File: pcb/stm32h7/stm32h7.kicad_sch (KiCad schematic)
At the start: 39 parts, among them J6 Test Pads, SW1 SW_Push, SW2 SW_Push, SW3 SW_Push, U1 STM32H743VGTx, U11 TPS61169DCKR, U9 MT25QUxxxxxx1xW7, Y1 25MHz

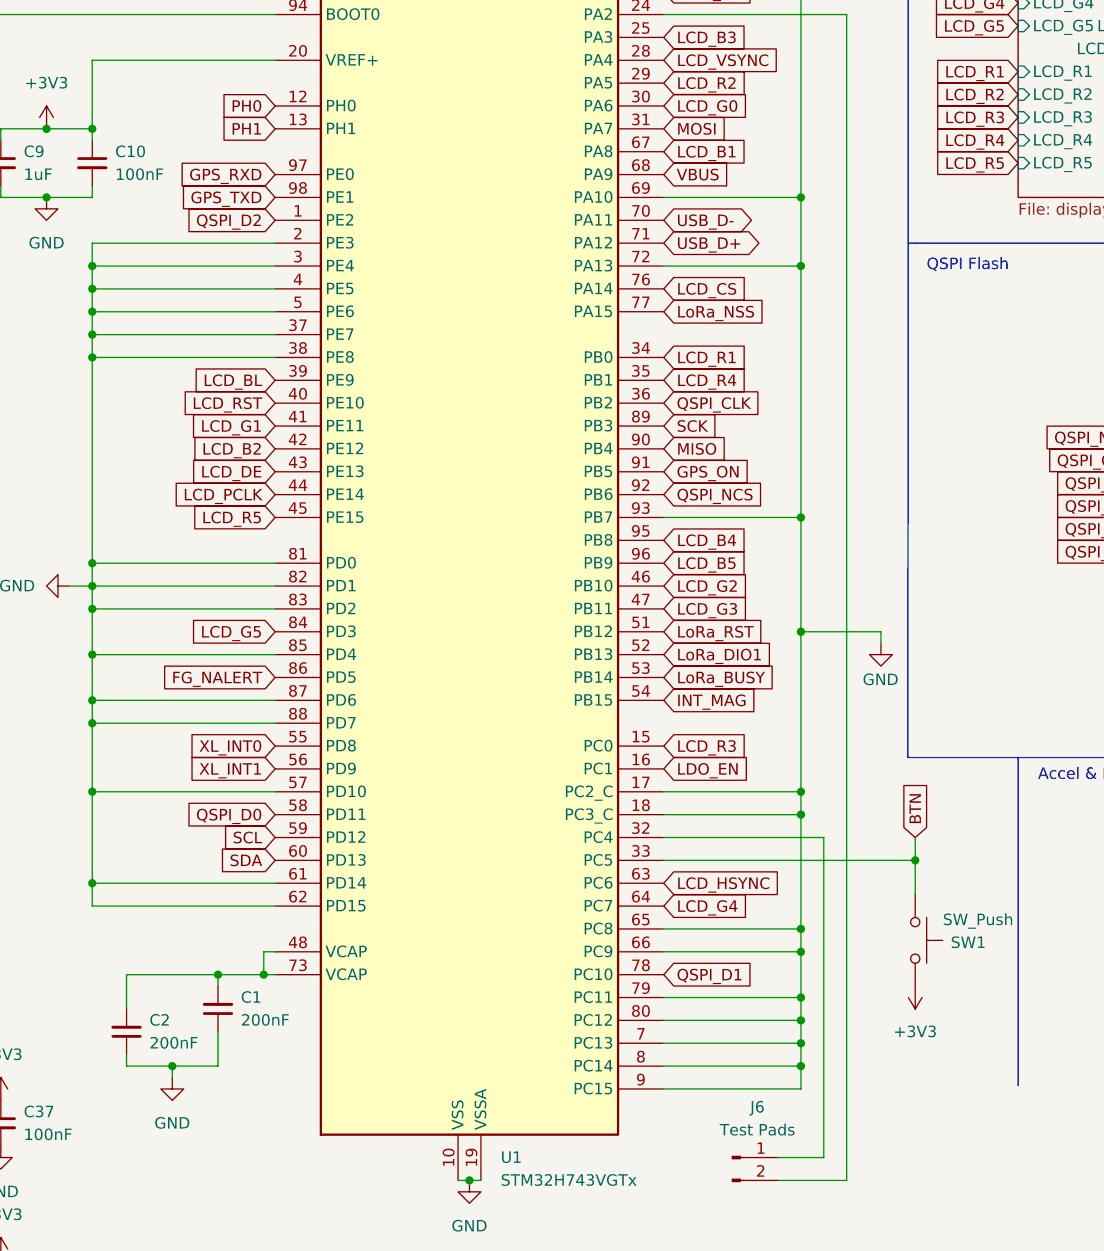
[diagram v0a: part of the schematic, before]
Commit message: everything is connected....
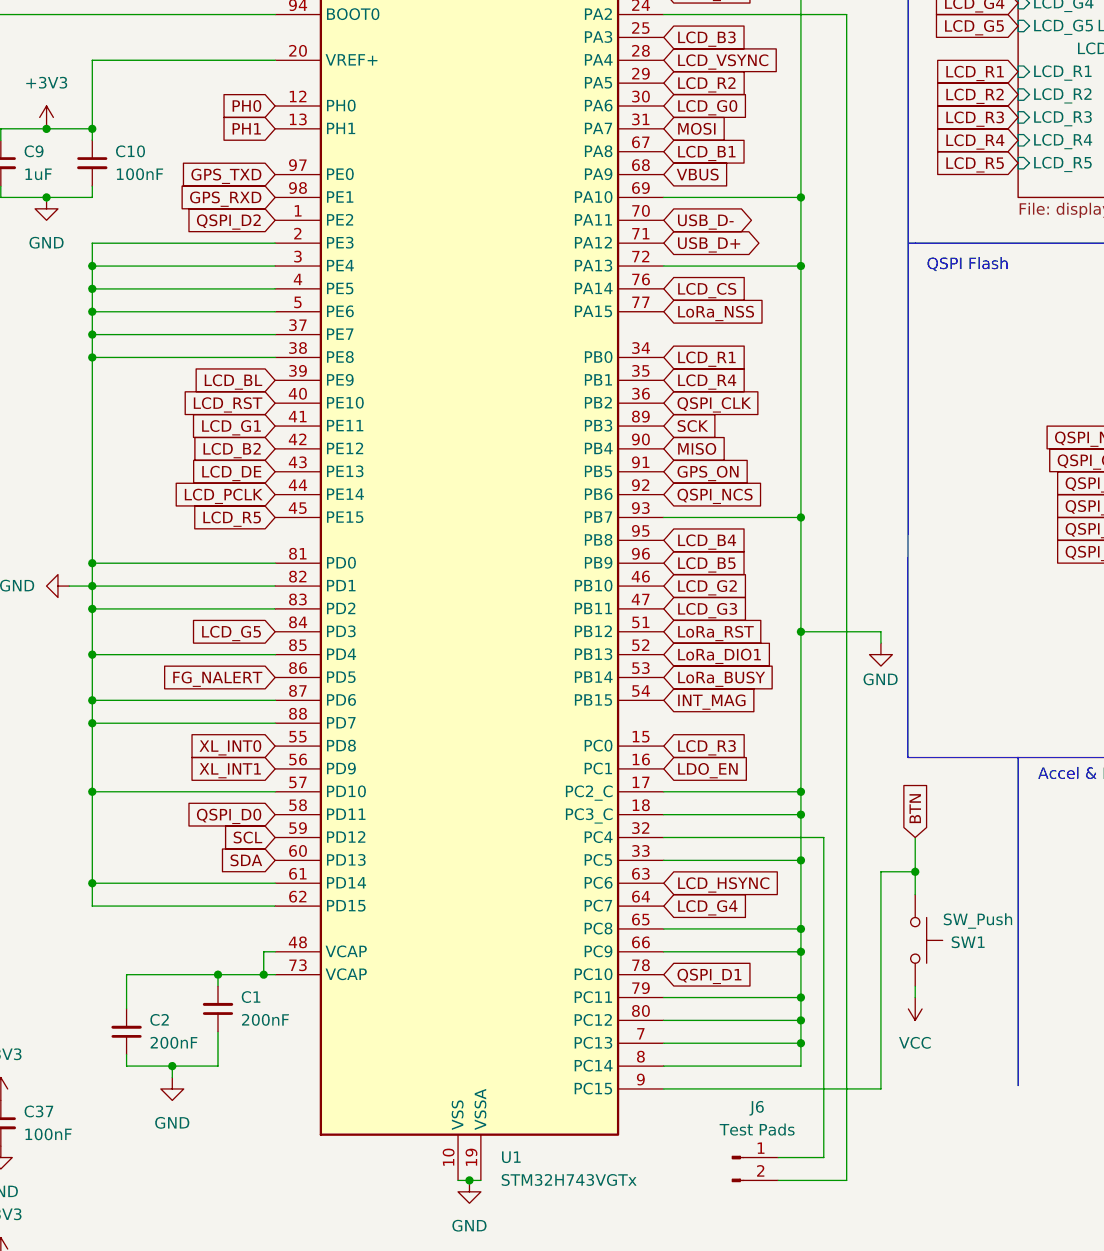
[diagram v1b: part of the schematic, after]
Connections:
- net +3V3: no longer SW1.2
- net BTN: now also U1.9 (PC15); no longer U1.33 (PC5)
- net GND: now also U1.33 (PC5); no longer U1.9 (PC15)
- net GPS_RXD: now also U1.98 (PE1); no longer U1.97 (PE0)
- net GPS_TXD: now also U1.97 (PE0); no longer U1.98 (PE1)
- net VCC: now also SW1.2
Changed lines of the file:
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@@
 	)
 	(junction
+		(at 177.8 142.24)
+		(diameter 0)
+		(color 0 0 0 0)
+	)
+	(junction
 		(at 156.21 185.42)
 		(diameter 0)
@@
 	)
 	(junction
-		(at 177.8 140.97)
-		(diameter 0)
-		(color 0 0 0 0)
-	)
-	(junction
-		(at 165.1 163.83)
-		(diameter 0)
-		(color 0 0 0 0)
-	)
-	(junction
 		(at 228.6 31.75)
 		(diameter 0)
@@
 	)
 	(junction
+		(at 165.1 140.97)
+		(diameter 0)
+		(color 0 0 0 0)
+	)
+	(junction
 		(at 86.36 110.49)
 		(diameter 0)
@@
 	(wire
 		(pts
-			(xy 149.86 166.37) (xy 165.1 166.37)
+			(xy 149.86 166.37) (xy 173.99 166.37)
 		)
 		(stroke
@@
 	(wire
 		(pts
-			(xy 165.1 135.89) (xy 165.1 148.59)
+			(xy 165.1 135.89) (xy 165.1 140.97)
 		)
 		(stroke
@@
 	(wire
 		(pts
+			(xy 173.99 142.24) (xy 177.8 142.24)
+		)
+		(stroke
+			(width 0)
+			(type default)
+		)
+	)
+	(wire
+		(pts
 			(xy 203.2 104.14) (xy 207.01 104.14)
 		)
@@
 		)
 	)
+	(wire
+		(pts
+			(xy 173.99 166.37) (xy 173.99 142.24)
+		)
+		(stroke
+			(width 0)
+			(type default)
+		)
+	)
 	(polyline
 		(pts
@@
 	(wire
 		(pts
-			(xy 177.8 140.97) (xy 177.8 138.43)
-		)
-		(stroke
-			(width 0)
-			(type default)
-		)
-	)
-	(wire
-		(pts
 			(xy 149.86 163.83) (xy 165.1 163.83)
 		)
@@
 	(wire
 		(pts
+			(xy 170.18 46.99) (xy 170.18 176.53)
+		)
+		(stroke
+			(width 0)
+			(type default)
+		)
+	)
+	(wire
+		(pts
 			(xy 165.1 102.87) (xy 165.1 115.57)
 		)
@@
 	(wire
 		(pts
-			(xy 149.86 140.97) (xy 177.8 140.97)
+			(xy 100.33 163.83) (xy 100.33 160.02)
 		)
 		(stroke
@@
 	(wire
 		(pts
-			(xy 100.33 163.83) (xy 100.33 160.02)
+			(xy 219.71 85.09) (xy 205.74 85.09)
 		)
 		(stroke
@@
 	(wire
 		(pts
-			(xy 219.71 85.09) (xy 205.74 85.09)
+			(xy 165.1 133.35) (xy 165.1 135.89)
 		)
 		(stroke
@@
 	(wire
 		(pts
-			(xy 165.1 133.35) (xy 165.1 135.89)
+			(xy 30.48 143.51) (xy 34.29 143.51)
 		)
 		(stroke
@@
 	(wire
 		(pts
-			(xy 30.48 143.51) (xy 34.29 143.51)
+			(xy 149.86 133.35) (xy 165.1 133.35)
 		)
 		(stroke
@@
 	(wire
 		(pts
-			(xy 149.86 133.35) (xy 165.1 133.35)
+			(xy 165.1 151.13) (xy 165.1 156.21)
 		)
 		(stroke
@@
 	(wire
 		(pts
-			(xy 165.1 151.13) (xy 165.1 156.21)
+			(xy 149.86 140.97) (xy 165.1 140.97)
 		)
 		(stroke
@@
 	(wire
 		(pts
-			(xy 177.8 144.78) (xy 177.8 140.97)
+			(xy 177.8 138.43) (xy 177.8 142.24)
 		)
 		(stroke
@@
 	(wire
 		(pts
-			(xy 170.18 46.99) (xy 170.18 176.53)
-		)
-		(stroke
-			(width 0)
-			(type default)
-		)
-	)
-	(wire
-		(pts
 			(xy 149.86 102.87) (xy 165.1 102.87)
 		)
@@
 		)
 	)
-	(wire
+	(polyline
 		(pts
-			(xy 165.1 163.83) (xy 165.1 166.37)
+			(xy 177.0288 12.0241) (xy 177.033 12.0241)
 		)
 		(stroke
@@
 		)
 	)
-	(polyline
+	(wire
 		(pts
-			(xy 177.0288 12.0241) (xy 177.033 12.0241)
+			(xy 149.86 41.91) (xy 165.1 41.91)
 		)
 		(stroke
@@
 	(wire
 		(pts
-			(xy 149.86 41.91) (xy 165.1 41.91)
+			(xy 25.4 80.01) (xy 34.29 80.01)
 		)
 		(stroke
@@
 	(wire
 		(pts
-			(xy 25.4 80.01) (xy 34.29 80.01)
+			(xy 124.46 21.59) (xy 124.46 34.29)
 		)
 		(stroke
@@
 	(wire
 		(pts
-			(xy 124.46 21.59) (xy 124.46 34.29)
+			(xy 165.1 140.97) (xy 165.1 148.59)
 		)
 		(stroke
@@
 	(wire
 		(pts
+			(xy 177.8 142.24) (xy 177.8 144.78)
+		)
+		(stroke
+			(width 0)
+			(type default)
+		)
+	)
+	(wire
+		(pts
 			(xy 153.67 24.13) (xy 153.67 21.59)
 		)
@@
 	(wire
 		(pts
+			(xy 177.8 156.21) (xy 177.8 154.94)
+		)
+		(stroke
+			(width 0)
+			(type default)
+		)
+	)
+	(wire
+		(pts
 			(xy 165.1 158.75) (xy 165.1 161.29)
 		)
@@
 	(global_label "GPS_TXD"
 		(shape input)
-		(at 106.68 67.31 180)
+		(at 106.68 64.77 180)
 		(fields_autoplaced yes)
 		(effects
@@
 		)
 		(property "Intersheetrefs" "${INTERSHEET_REFS}"
-			(at 95.5306 67.31 0)
+			(at 95.5306 64.77 0)
 			(effects
 				(font
@@
 	(global_label "GPS_RXD"
 		(shape input)
-		(at 106.68 64.77 180)
+		(at 106.68 67.31 180)
 		(fields_autoplaced yes)
 		(effects
@@
 		)
 		(property "Intersheetrefs" "${INTERSHEET_REFS}"
-			(at 95.2282 64.77 0)
+			(at 95.2282 67.31 0)
 			(effects
 				(font
@@
 	)
 	(symbol
+		(lib_id "power:VCC")
+		(at 177.8 156.21 180)
+		(unit 1)
+		(exclude_from_sim no)
+		(in_bom yes)
+		(on_board yes)
+		(dnp no)
+		(fields_autoplaced yes)
+		(property "Reference" "#PWR069"
+			(at 177.8 152.4 0)
+			(effects
+				(font
+					(size 1.27 1.27)
+				)
+				(hide yes)
+			)
+		)
+		(property "Value" "VCC"
+			(at 177.8 161.29 0)
+			(effects
+				(font
+					(size 1.27 1.27)
+				)
+			)
+		)
+		(property "Footprint" ""
+			(at 177.8 156.21 0)
+			(effects
+				(font
+					(size 1.27 1.27)
+				)
+				(hide yes)
+			)
+		)
+		(property "Datasheet" ""
+			(at 177.8 156.21 0)
+			(effects
+				(font
+					(size 1.27 1.27)
+				)
+				(hide yes)
+			)
+		)
+		(property "Description" "Power symbol creates a global label with name \"VCC\""
+			(at 177.8 156.21 0)
+			(effects
+				(font
+					(size 1.27 1.27)
+				)
+				(hide yes)
+			)
+		)
+		(pin "1"
+		)
+		(instances
+			(project "stm32h7"
+				(path "/834edf73-57a5-43b4-ab36-0b077e93e6d5"
+					(reference "#PWR069")
+					(unit 1)
+				)
+			)
+		)
+	)
+	(symbol
 		(lib_id "power:+3V3")
 		(at 124.46 20.32 0)
@@
 					(unit 1)
 				)
-			)
-		)
-	)
-	(symbol
-		(lib_id "power:+3V3")
-		(at 177.8 154.94 180)
-		(unit 1)
-		(exclude_from_sim no)
-		(in_bom yes)
-		(on_board yes)
-		(dnp no)
-		(fields_autoplaced yes)
-		(property "Reference" "#PWR069"
-			(at 177.8 151.13 0)
-			(effects
-				(font
-					(size 1.27 1.27)
-				)
-				(hide yes)
-			)
-		)
-		(property "Value" "+3V3"
-			(at 177.8 160.02 0)
-			(effects
-				(font
-					(size 1.27 1.27)
-				)
-			)
-		)
-		(property "Footprint" ""
-			(at 177.8 154.94 0)
-			(effects
-				(font
-					(size 1.27 1.27)
-				)
-				(hide yes)
-			)
-		)
-		(property "Datasheet" ""
-			(at 177.8 154.94 0)
-			(effects
-				(font
-					(size 1.27 1.27)
-				)
-				(hide yes)
-			)
-		)
-		(property "Description" "Power symbol creates a global label with name \"+3V3\""
-			(at 177.8 154.94 0)
-			(effects
-				(font
-					(size 1.27 1.27)
-				)
-				(hide yes)
-			)
-		)
-		(pin "1"
-		)
-		(instances
-			(project "stm32h7"
-				(path "/834edf73-57a5-43b4-ab36-0b077e93e6d5"
-					(reference "#PWR069")
-					(unit 1)
-				)
